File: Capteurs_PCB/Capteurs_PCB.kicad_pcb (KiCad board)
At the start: 2 copper layers, 51 x 70 mm, 59 parts, among them J1 Conn_01x04, J101 Conn_01x03, J103 Conn_02x20_Odd_Even, J104 Conn_ST_STDC14, J2 Conn_01x03, J3 Alim_Prop2, J4 Conn_01x02, J5 Alim_Prop1, J6 Conn_01x03, J7 Conn_01x03, U1 STM32L412KBTx, U3 LSM6DSL, U6 32350268

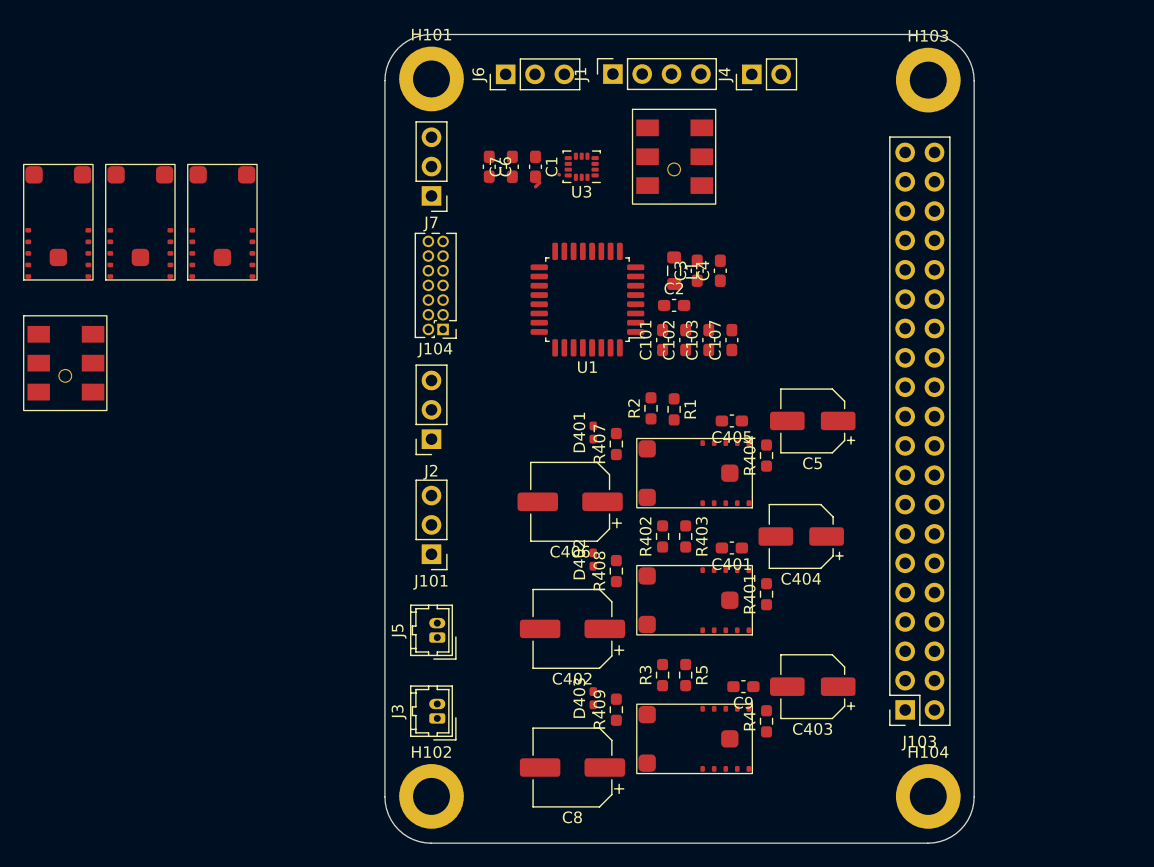
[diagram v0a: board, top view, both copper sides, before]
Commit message: Début de routage
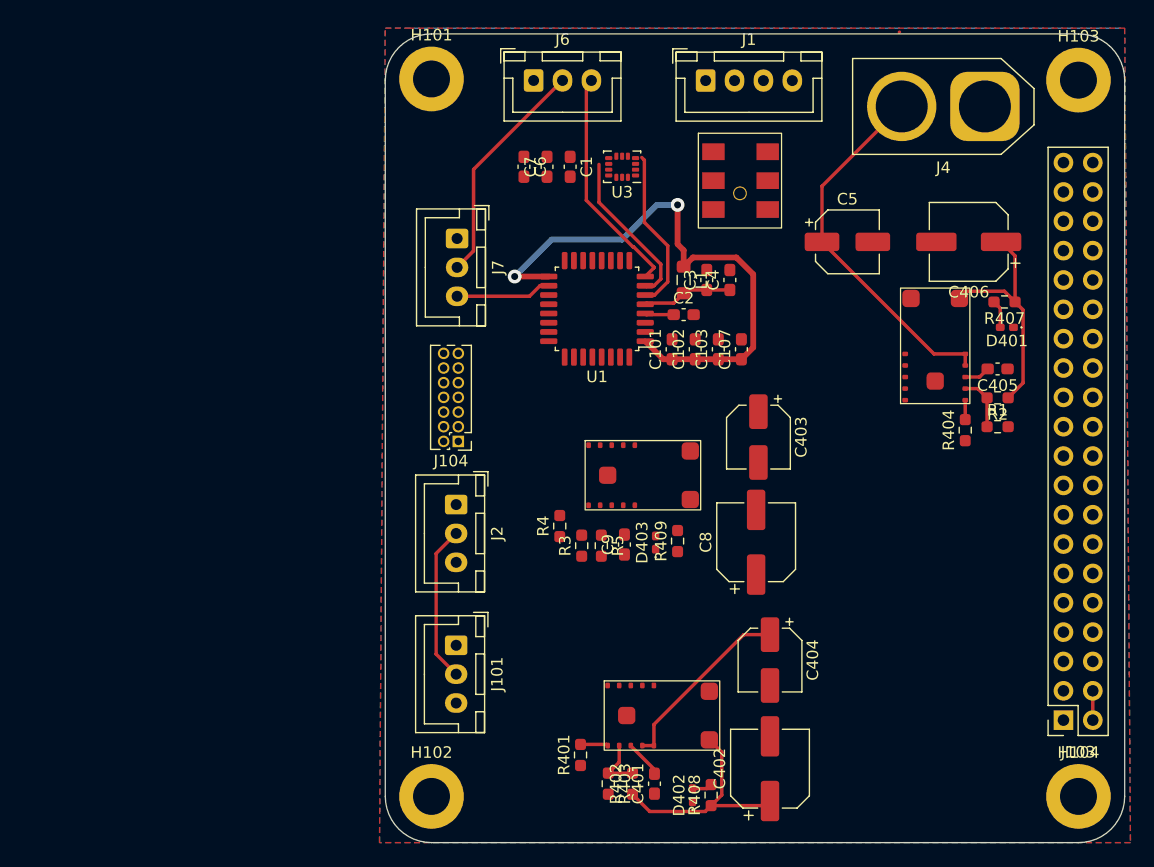
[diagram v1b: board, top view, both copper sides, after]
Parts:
- removed J3: Alim_Prop2, Connector_Hirose:Hirose_DF13-02P-1.25DSA_1x02_P1.25mm_Vertical
- removed J5: Alim_Prop1, Connector_Hirose:Hirose_DF13-02P-1.25DSA_1x02_P1.25mm_Vertical
- removed the U2 at (127.8, 110.5)
- removed the U401 at (127.8, 98.5)
- removed the U402 at (127.8, 87.5)
- removed the U6 at (126.0, 60.1)
- J1: footprint Connector_PinSocket_2.54mm:PinSocket_1x04_P2.54mm_Vertical -> Connector_JST:JST_XH_B4B-XH-A_1x04_P2.50mm_Vertical
- J101, J6, J7: footprint Connector_PinHeader_2.54mm:PinHeader_1x03_P2.54mm_Vertical -> Connector_JST:JST_XH_B3B-XH-A_1x03_P2.50mm_Vertical
- J2: footprint Connector_PinSocket_2.54mm:PinSocket_1x03_P2.54mm_Vertical -> Connector_JST:JST_XH_B3B-XH-A_1x03_P2.50mm_Vertical
- J4: footprint Connector_PinHeader_2.54mm:PinHeader_1x02_P2.54mm_Vertical -> Connector_AMASS:AMASS_XT60-M_1x02_P7.20mm_Vertical
- moved U402 62.6 mm to (148.6, 76.5)
- moved U401 62.1 mm to (125.0, 108.5), turned to -90 degrees
- moved U6 60.5 mm to (131.7, 62.2)
- moved U2 55.1 mm to (123.3, 87.7), turned to -90 degrees
- moved C406 41.2 mm to (151.5, 67.5)
- moved D401 36.9 mm to (154.8, 74.9), turned to 180 degrees
- moved R407 35.8 mm to (154.6, 72.7), turned to 180 degrees
- moved R2 30.0 mm to (154.0, 81.0), turned to 180 degrees
- moved R1 28.0 mm to (154.0, 83.5), turned to 0 degrees
- moved C8 25.2 mm to (133.1, 93.5), turned to 90 degrees
- moved R4 24.6 mm to (116.1, 92.1)
- moved C405 23.4 mm to (154.0, 78.5)
- moved R403 22.4 mm to (120.3, 114.4)
- moved D402 22.1 mm to (127.6, 115.4)
- moved C403 22.1 mm to (133.3, 84.4), turned to -90 degrees
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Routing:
- net +3.3V: track 0.02 -> 48.9 mm, vias 0 -> 2
- net +BATT: track 0.00 -> 48.1 mm
- net +5V: track 0.00 -> 35.6 mm
- net +7.5V: track 0.00 -> 20.3 mm
- net /VDD_SER: track 0.00 -> 20.0 mm
- net /DATA1: track 0.00 -> 19.9 mm
- net /INT1: track 0.00 -> 14.1 mm
- net /INT2: track 0.00 -> 13.9 mm
- net /DATA2: track 0.00 -> 8.31 mm
- net +3.3VA: track 0.00 -> 7.84 mm
- net Net-(U401-FB): track 0.00 -> 4.88 mm
- net Net-(U402-FB): track 0.00 -> 4.72 mm
- net Net-(U401-Vcc): track 0.00 -> 3.29 mm
- net /NRST: track 0.00 -> 2.50 mm
- net Net-(D401-A): track 0.00 -> 2.42 mm
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- added copper zone on B.Cu, net GND
- added copper zone on F.Cu, net GND
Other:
- board size 51 x 70 mm -> 64 x 70 mm
